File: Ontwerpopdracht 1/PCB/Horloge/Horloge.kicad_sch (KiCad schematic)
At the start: 37 parts, among them J1 Conn_01x01, J1 Conn_01x03, J2 Conn_01x01, Q1 BSS138, U1 ATTINY1614-SSF, U1 TPS613222ADBVT, Y1 FX135A-327

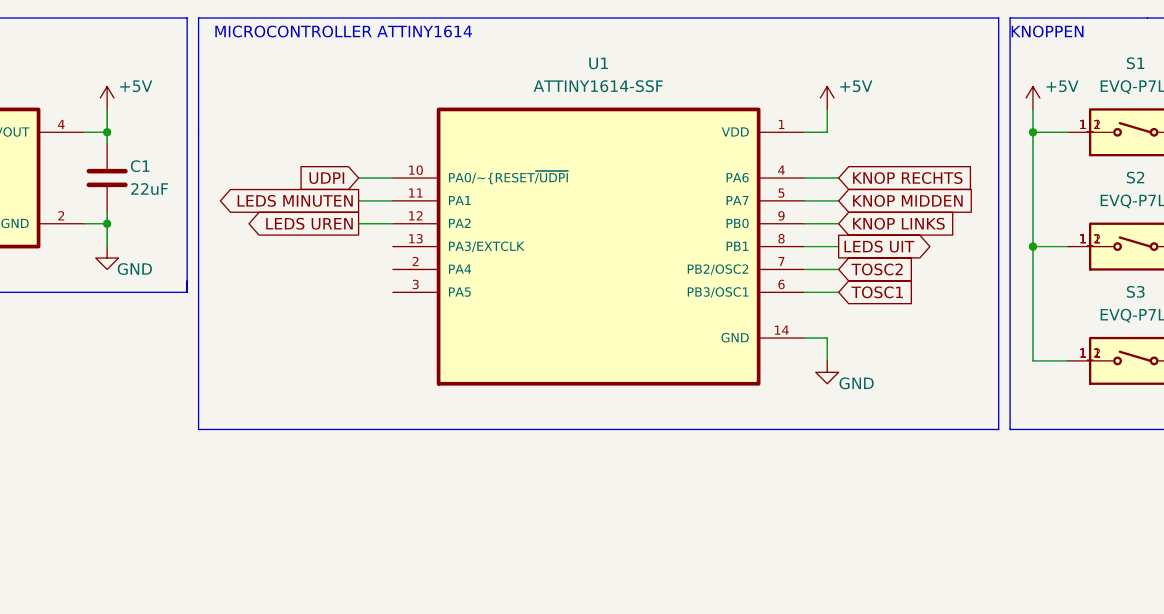
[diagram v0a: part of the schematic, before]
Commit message: aanpassing attiny, update doc schema
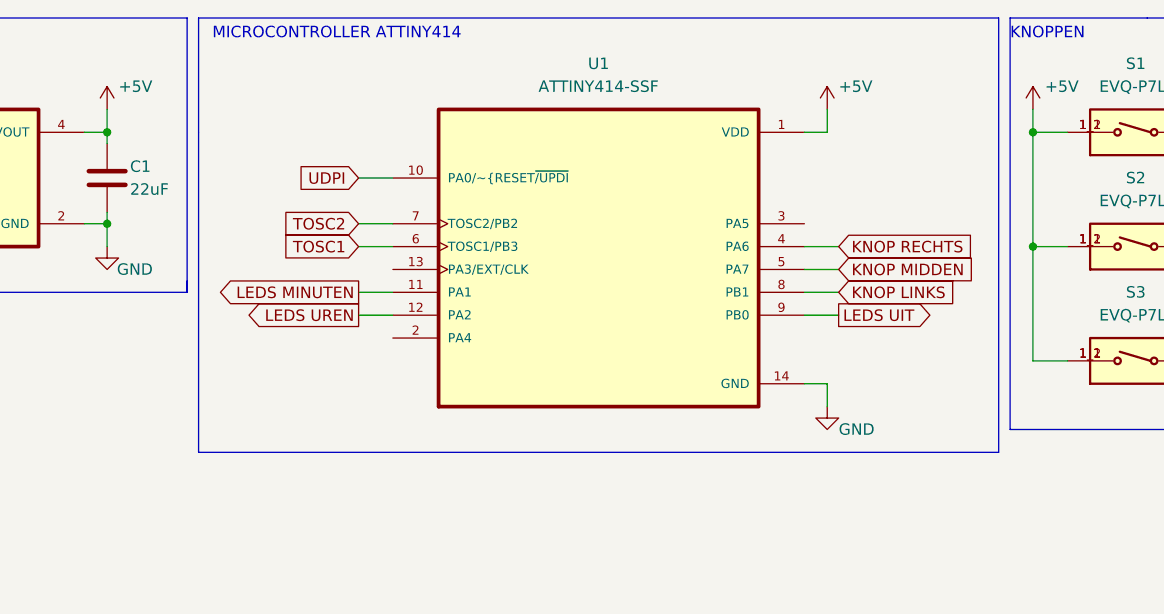
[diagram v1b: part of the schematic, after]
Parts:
- removed U1: ATTINY1614-SSF, ATTINY1614-SSF:SOIC127P600X175-14N, symbol ATTINY1614-SSF:ATTINY1614-SSF
- added U1: ATTINY414-SSF, SOIC127P600X175-14N, symbol ATTINY414-SSF:ATTINY414-SSF
- C1: footprint (none) -> GRM21BR61A226ME51L:CAPC2012X140N
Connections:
- net +5V: now also U1.1 (VDD)
- net GND: now also U1.14 (GND)
- net KNOP LINKS: now also U1.8 (PB1)
- net KNOP MIDDEN: now also U1.5 (PA7)
- net KNOP RECHTS: now also U1.4 (PA6)
- net LEDS MINUTEN: now also U1.11 (PA1)
- net LEDS UIT: now also U1.9 (PB0)
- net LEDS UREN: now also U1.12 (PA2)
- net TOSC1: now also U1.6 (TOSC1/PB3)
- net TOSC2: now also U1.7 (TOSC2/PB2)
- net UDPI: now also U1.10 (PA0/~{RESET~{/UPDI})
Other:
- note added: "MICROCONTROLLER ATTINY414"
- note removed: "MICROCONTROLLER ATTINY1614"

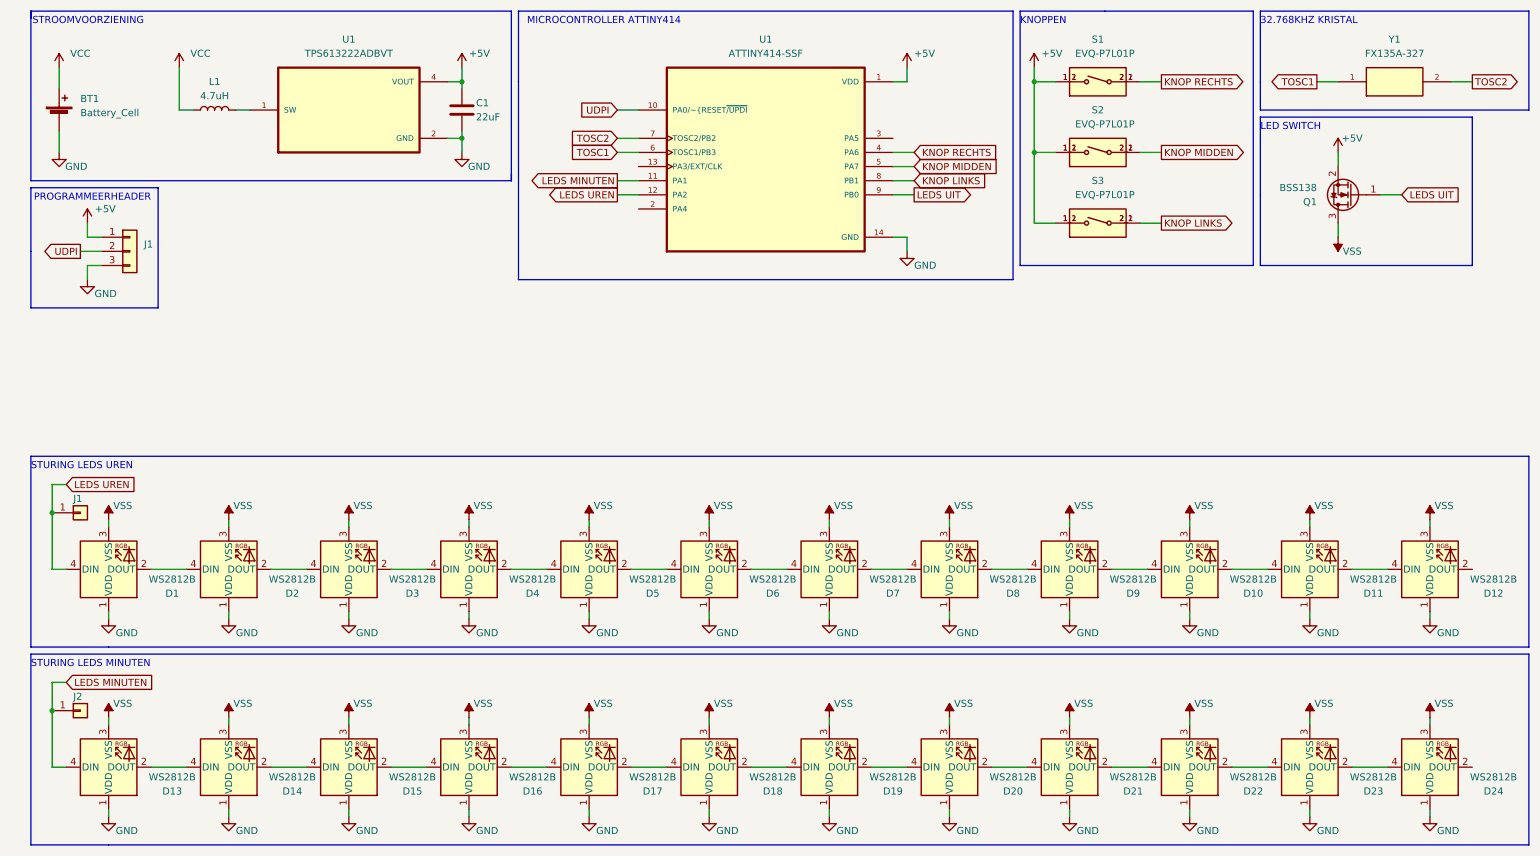
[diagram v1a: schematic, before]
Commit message: aanpassing schema
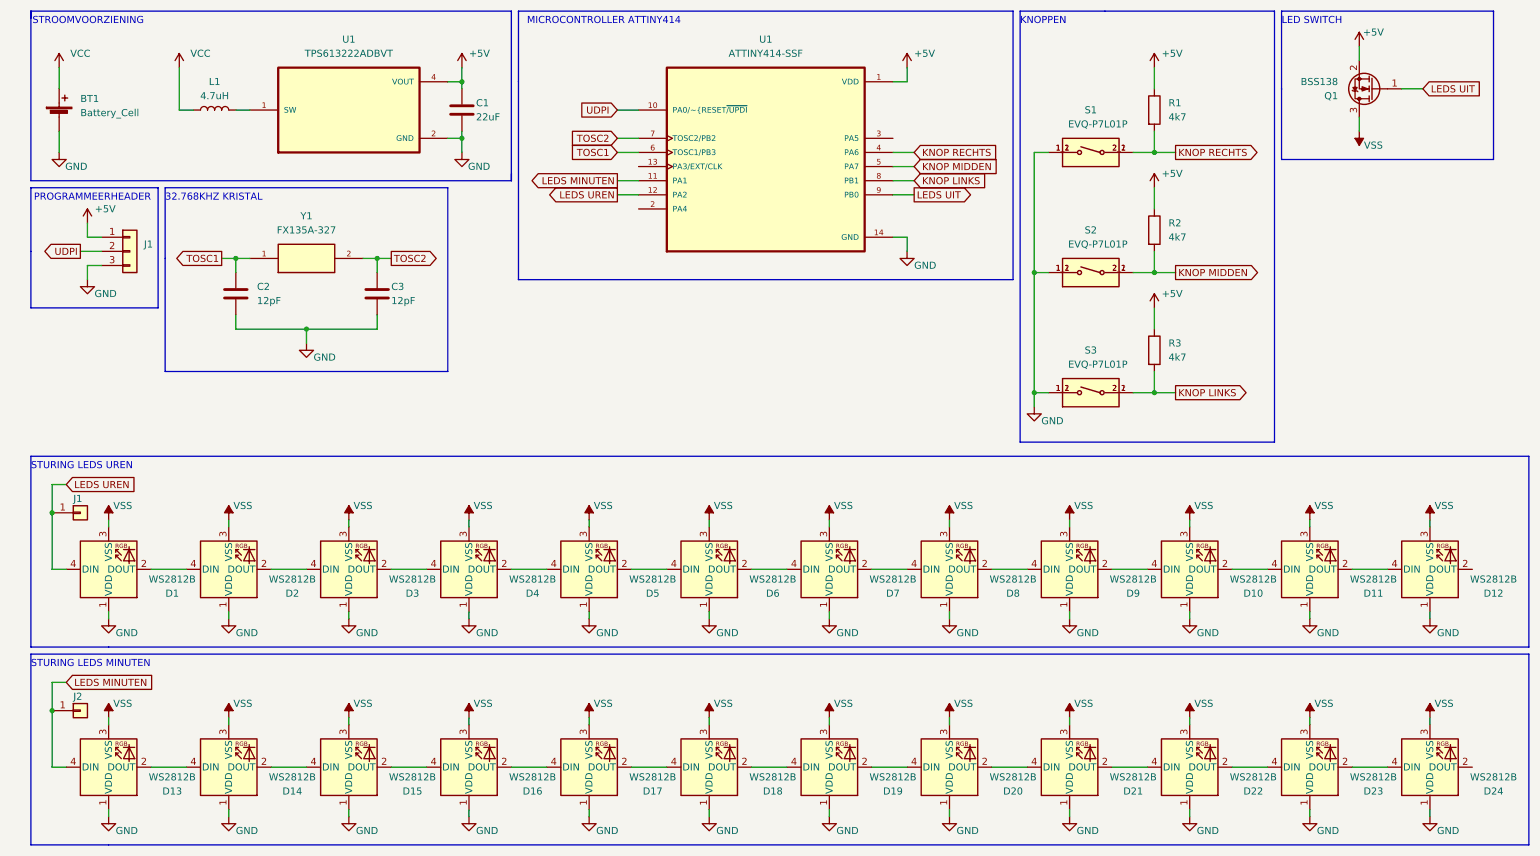
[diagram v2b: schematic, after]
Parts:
- added C2, C3: 12pF, GRM21BR61A226ME51L:CAPC2012X140N, symbol Device:C
- added R1, R2, R3: 4k7, symbol Device:R
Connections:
- net +5V: now also R1.1, R2.1, R3.1; no longer S1.1_1, S1.1_2, S2.1_1, S2.1_2, S3.1_1, S3.1_2
- net GND: now also S1.1_1, S1.1_2, S2.1_1, S2.1_2, S3.1_1, S3.1_2, C2.2, C3.2
- net KNOP LINKS: now also R3.2
- net KNOP MIDDEN: now also R2.2
- net KNOP RECHTS: now also R1.2
- net TOSC1: now also C2.1
- net TOSC2: now also C3.1
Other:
- moved on the sheet: Q1, S1, S2, S3, Y1
